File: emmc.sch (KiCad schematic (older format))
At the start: 30 parts

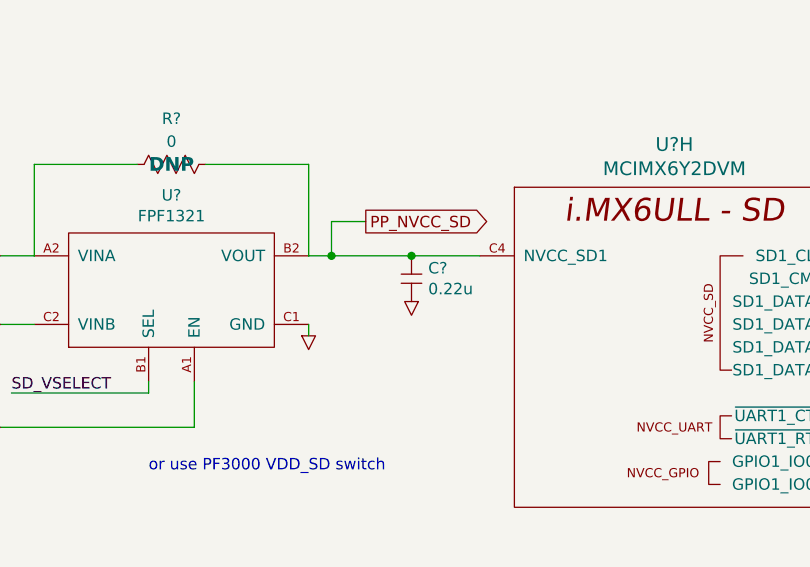
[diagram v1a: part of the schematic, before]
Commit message: start some usb
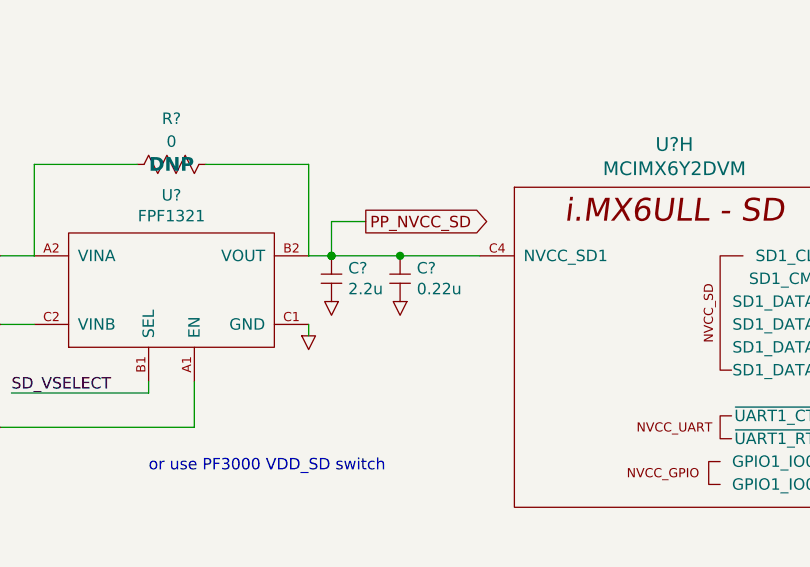
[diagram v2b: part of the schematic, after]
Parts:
- added C?: 2.2u, symbol C
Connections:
- net COM: now also C?.2
- net PP_NVCC_SD: now also C?.1
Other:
- moved on the sheet: C?
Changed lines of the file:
@@
 L C C?
 U 1 1 5A0CF3A2
-P 3000 5200
-F 0 "C?" H 3073 5146 50  0000 L CNN
-F 1 "0.22u" H 3073 5055 50  0000 L CNN
-F 2 "" H 2900 5350 60  0000 C CNN
-F 3 "" H 2900 5350 60  0000 C CNN
-	1    3000 5200
+P 2950 5200
+F 0 "C?" H 3023 5146 50  0000 L CNN
+F 1 "0.22u" H 3023 5055 50  0000 L CNN
+F 2 "" H 2850 5350 60  0000 C CNN
+F 3 "" H 2850 5350 60  0000 C CNN
+	1    2950 5200
 	1    0    0    -1
 $EndComp
@@
 L COM #PWR?
 U 1 1 5A0CF3B0
-P 3000 5400
-F 0 "#PWR?" V 3275 5400 60  0001 C CNN
-F 1 "COM" H 3160 5285 30  0001 C CNN
-F 2 "" H 3155 5410 60  0000 C CNN
-F 3 "" H 3155 5410 60  0000 C CNN
-	1    3000 5400
+P 2950 5400
+F 0 "#PWR?" V 3225 5400 60  0001 C CNN
+F 1 "COM" H 3110 5285 30  0001 C CNN
+F 2 "" H 3105 5410 60  0000 C CNN
+F 3 "" H 3105 5410 60  0000 C CNN
+	1    2950 5400
 	-1   0    0    -1
 $EndComp
@@
 	2550 5200 2650 5200
 Wire Wire Line
-	2650 5200 3000 5200
-Wire Wire Line
-	3000 5200 3300 5200
+	2650 5200 2650 5200
+Wire Wire Line
+	2650 5200 2950 5200
+Wire Wire Line
+	2950 5200 3300 5200
 Wire Wire Line
 	2550 5500 2550 5500
@@
 Wire Wire Line
 	2050 5950 2050 5750
-Connection ~ 3000 5200
+Connection ~ 2950 5200
 Wire Wire Line
 	9150 4650 9800 4650
@@
 Wire Wire Line
 	5700 6750 5700 6800
+$Comp
+L C C?
+U 1 1 5A12F565
+P 2650 5200
+F 0 "C?" H 2723 5146 50  0000 L CNN
+F 1 "2.2u" H 2723 5055 50  0000 L CNN
+F 2 "" H 2550 5350 60  0000 C CNN
+F 3 "" H 2550 5350 60  0000 C CNN
+	1    2650 5200
+	1    0    0    -1
+$EndComp
+$Comp
+L COM #PWR?
+U 1 1 5A12F56C
+P 2650 5400
+F 0 "#PWR?" V 2925 5400 60  0001 C CNN
+F 1 "COM" H 2810 5285 30  0001 C CNN
+F 2 "" H 2805 5410 60  0000 C CNN
+F 3 "" H 2805 5410 60  0000 C CNN
+	1    2650 5400
+	-1   0    0    -1
+$EndComp
+Connection ~ 2650 5200
 $EndSCHEMATC

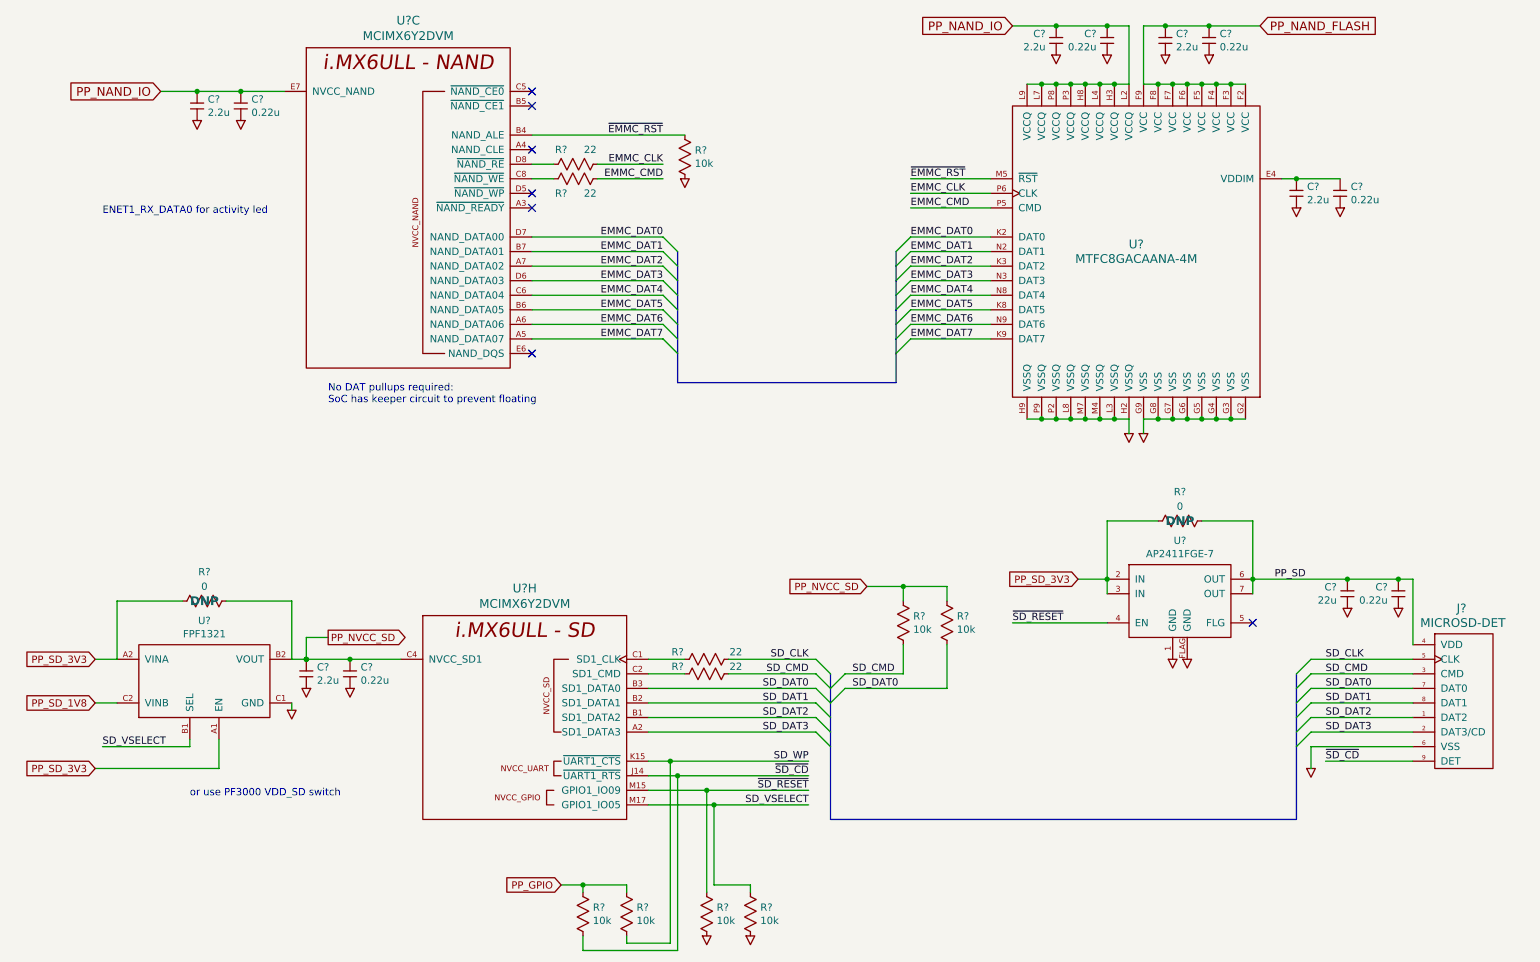
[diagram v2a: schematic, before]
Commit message: schematic progress
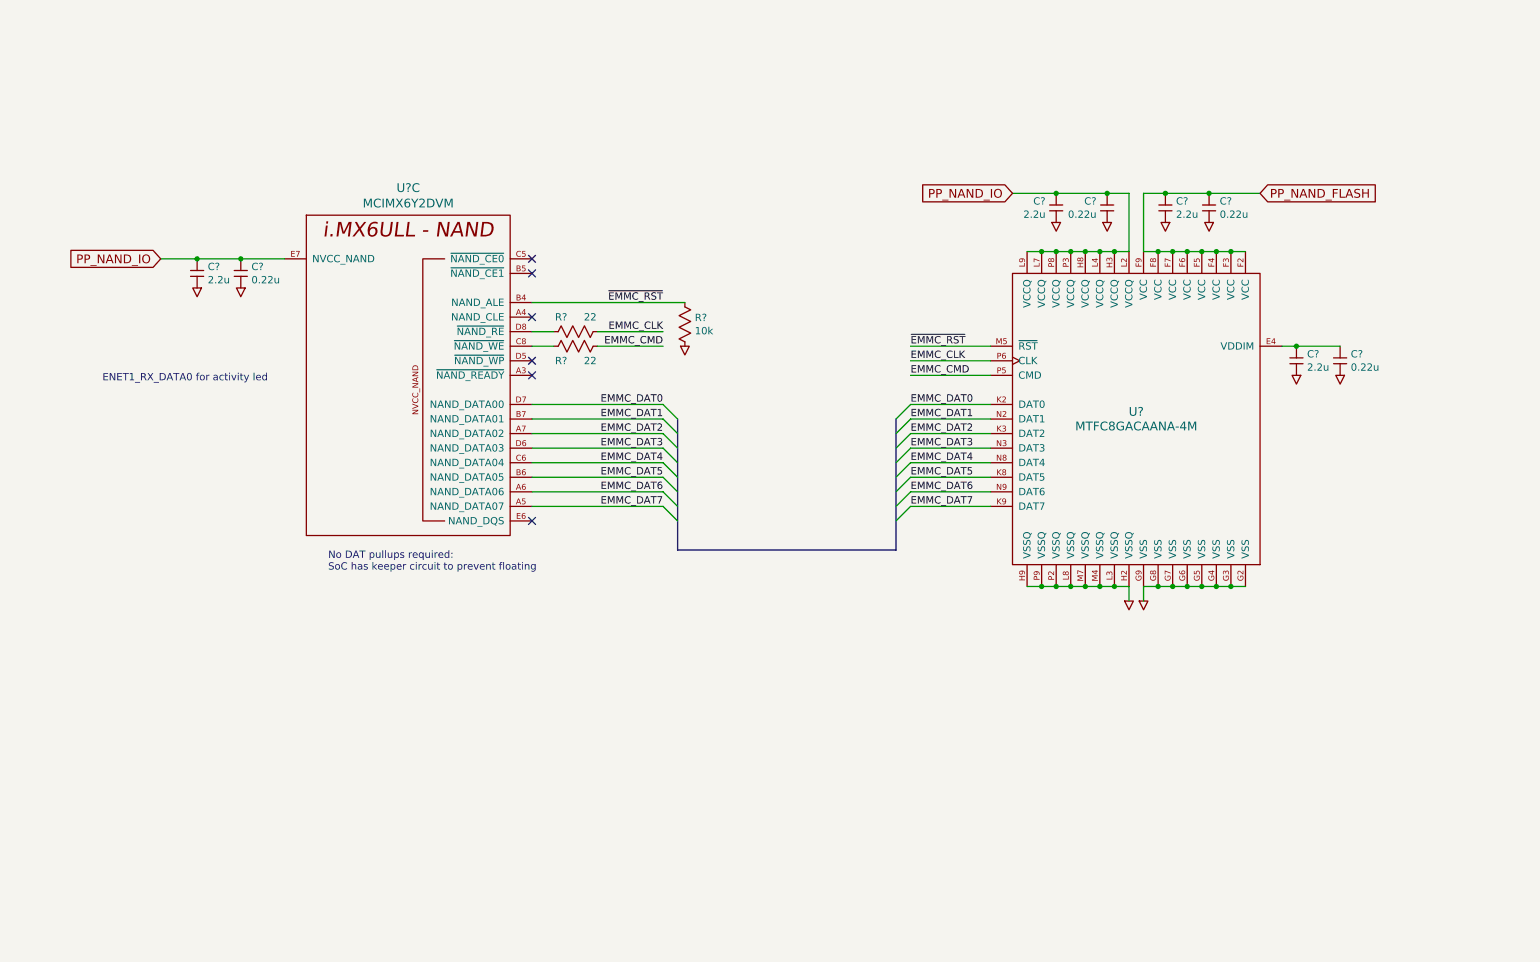
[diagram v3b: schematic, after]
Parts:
- removed C? (x2): 0.22u, symbol C
- removed C?: 22u, symbol C
- removed C?: 2.2u, symbol C
- removed J?: MICROSD-DET, symbol MICROSD-DET
- removed R? (x6): 10k, symbol R
- removed R? (x2): 22, symbol R
- removed R? (x2): 0, symbol R
- removed U?: MCIMX6Y2DVM, symbol MCIMX6Y2DVM
- removed U?: FPF1321, symbol FPF1321
- removed U?: AP2411FGE-7, symbol AP24x1-U-DFN3030
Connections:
- no-connect marks 7 -> 6
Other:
- note removed: "or use PF3000 VDD_SD switch"
- moved on the sheet: C?, R?, U?, U?C

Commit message: power design
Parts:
- C401, C403, C405, C407: renamed from C?; value 2.2u -> 10u; footprint (none) -> kicad-libs:SMD-1005; symbol C -> c:C; Manufacturer (none) -> Murata; Part Number (none) -> GRM155R60G106ME44D
- C402, C404, C406, C408: renamed from C?; footprint (none) -> kicad-libs:SMD-1005; symbol C -> c:C; Manufacturer (none) -> Samsung; Part Number (none) -> CL05B224KQ5NNWC
- R401, R402, R403: renamed from R?; symbol R -> r:R
- U201: renamed from U?; symbol MCIMX6Y2DVM -> mcimx6y2dvm:MCIMX6Y2DVM
- U401: renamed from U?; symbol eMMC-100FBGA -> emmc-100fbga:eMMC-100FBGA
